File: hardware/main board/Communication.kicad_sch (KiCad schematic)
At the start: 14 parts, among them U3 MCP2542FDxMF, U4 USBLC6-2SC6, U6 MCP2542FDxMF

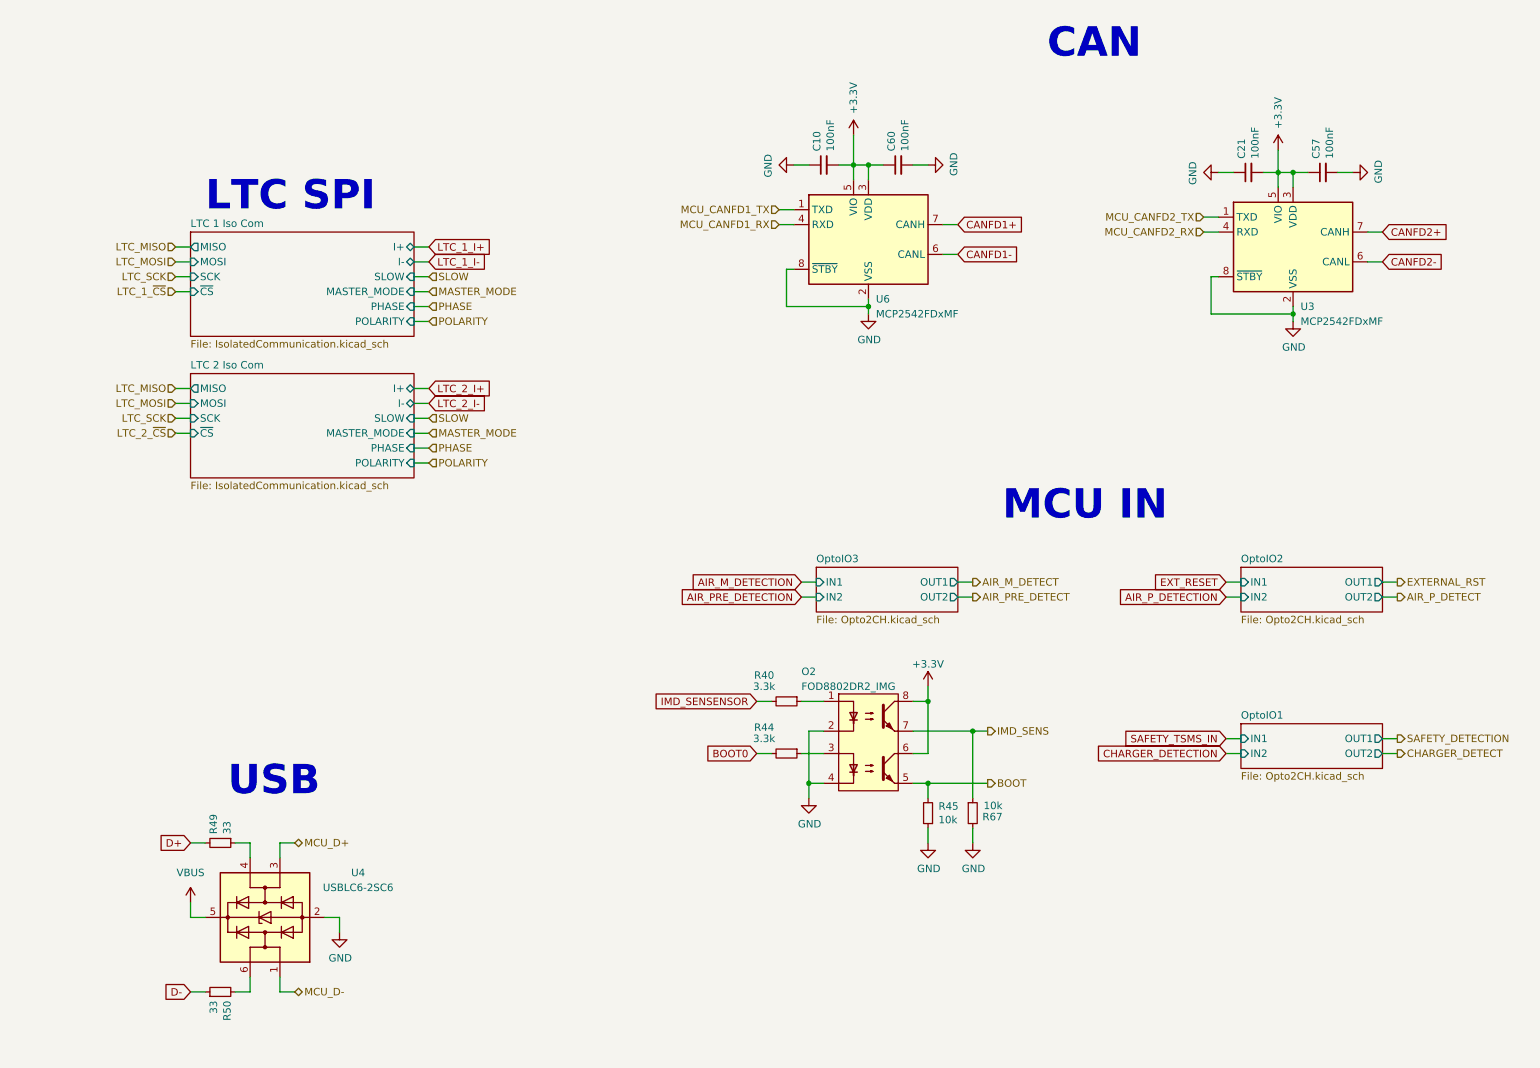
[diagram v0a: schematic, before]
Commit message: repairing demaged branch~
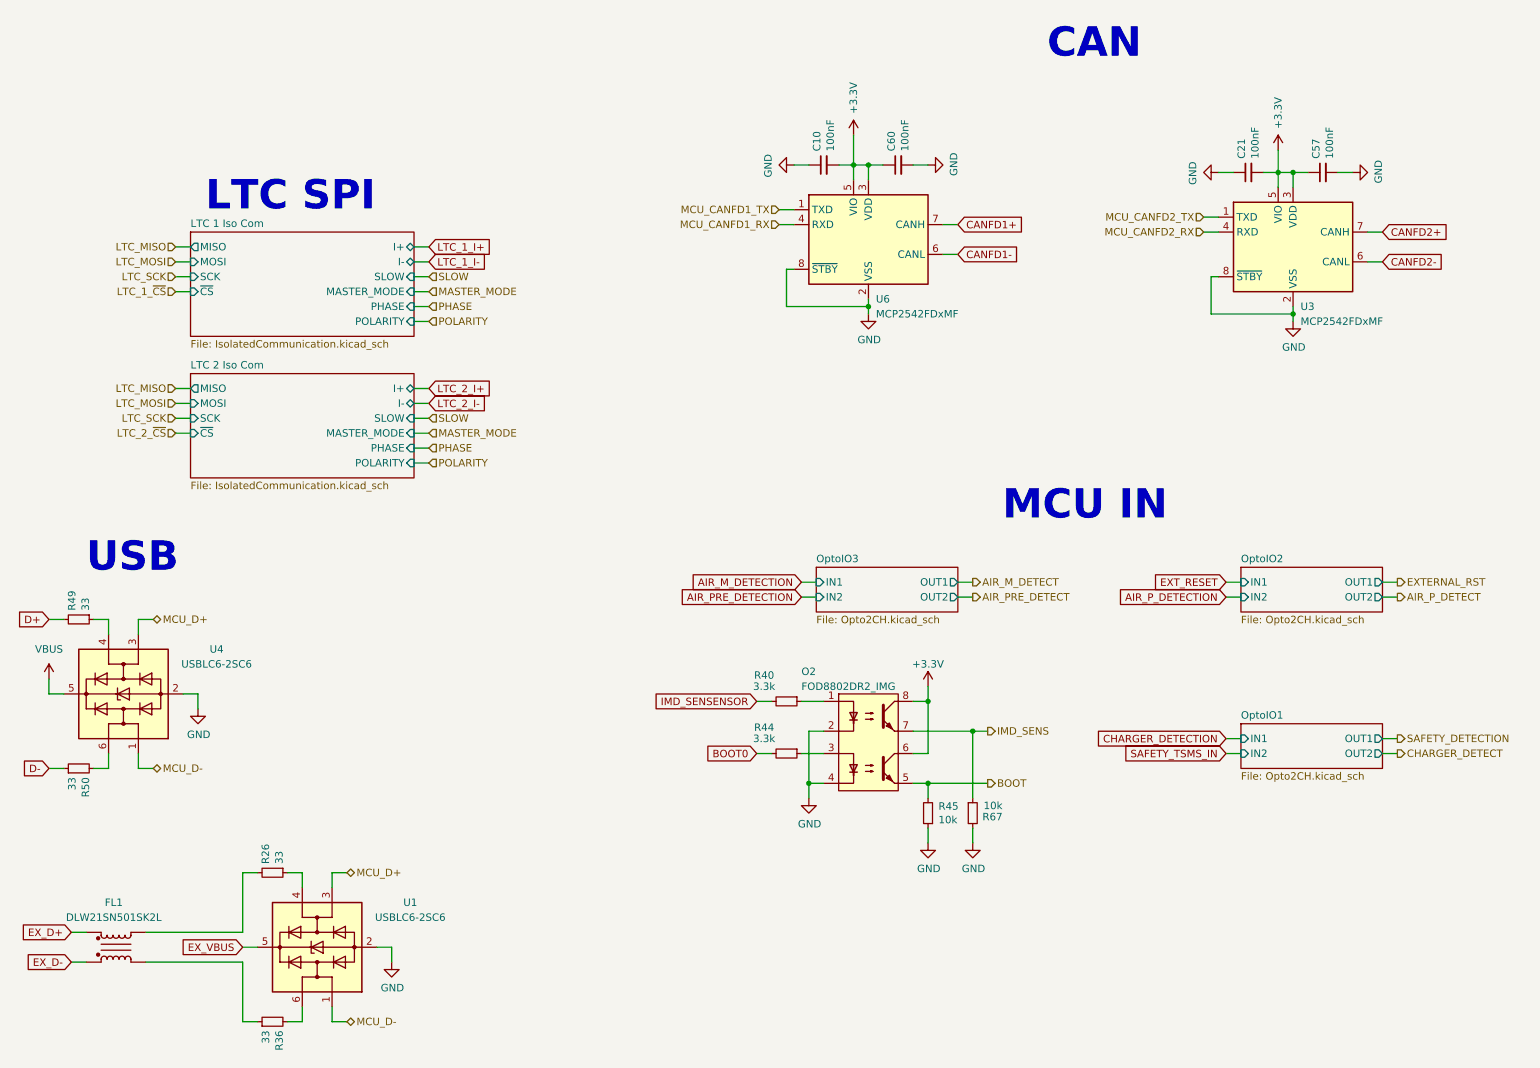
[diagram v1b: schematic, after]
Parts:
- added FL1: DLW21SN501SK2L, Samacsys:DLW21SN121HQ2L, symbol dlw21sn501sk2l:DLW21SN501SK2L
- added R26, R36: 33, Resistor_SMD:R_0603_1608Metric, symbol Device:R_Small
- added U1: USBLC6-2SC6, Package_TO_SOT_SMD:SOT-23-6, symbol Power_Protection:USBLC6-2SC6
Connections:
- net GND: now also U1.2 (GND)
- net MCU_D+: now also U1.3 (I/O2)
- net MCU_D-: now also U1.1 (I/O1)
- new net: FL1.2, R36.1
- new net: FL1.3, R26.2
- new net: R26.1, U1.4 (I/O2)
- new net: R36.2, U1.6 (I/O1)
- new net EX_D+: FL1.4
- new net EX_D-: FL1.1
- new net EX_VBUS: U1.5 (VBUS)
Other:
- moved on the sheet: R49, R50, U4
